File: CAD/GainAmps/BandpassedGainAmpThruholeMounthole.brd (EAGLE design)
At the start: 10.7 x 26.9 mm, 9 parts, among them U1 OPA202IDR

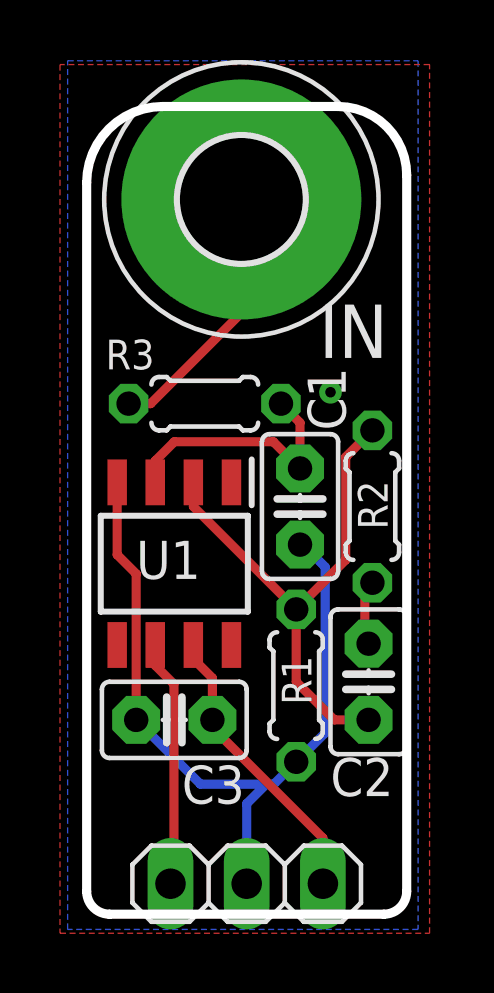
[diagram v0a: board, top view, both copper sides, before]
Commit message: fixes
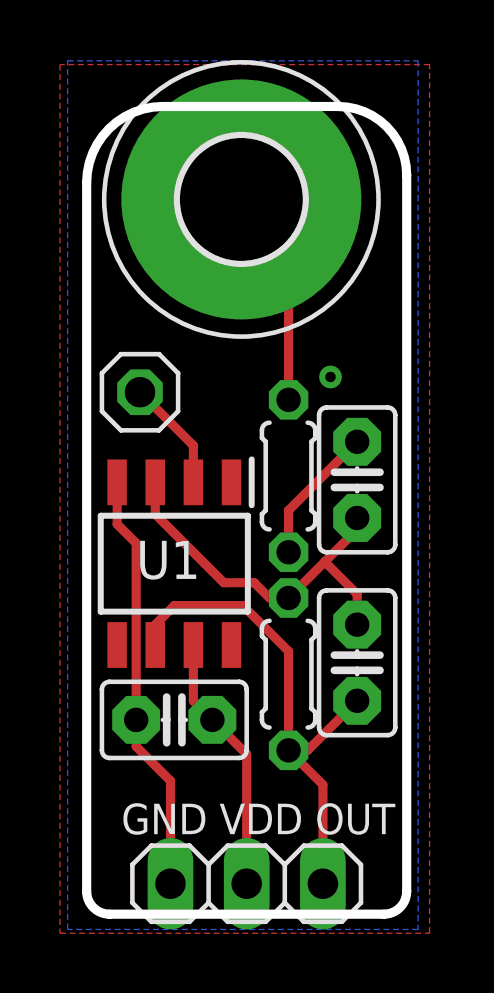
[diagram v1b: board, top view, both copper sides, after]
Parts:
- removed R3: 1K, rcl:0204/5
- added REF: (no value), pinhead:1X01
- moved R1 6.99 mm to (7.75, 17.7), turned to 270 degrees
- moved R2 6.25 mm to (7.75, 11.0)
- moved C1 2.10 mm to (10.0, 17.5), turned to 270 degrees
- moved C2 0.74 mm to (10.0, 11.4), turned to 270 degrees
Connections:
- removed net -IN: C2.1, R1.2, R2.1, U1.2
- removed net N$3: C2.2, R2.2
- new net +REF: REF.1, U1.2
- new net R1C1: C1.1, R1.2
- net +IN: now also C2.1, R2.1; no longer R3.2
- net GND: now also JP1.3; no longer C1.1, JP1.2, R1.1
- net IN: now also R1.1; no longer R3.1
- net OUT: now also C2.2, JP1.1, R2.2; no longer JP1.3
- net VDD: now also JP1.2; no longer JP1.1
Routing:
- net -IN: track 18.0 -> 0.00 mm
- net GND: track 26.3 -> 14.1 mm
- net OUT: track 8.29 -> 17.2 mm
- net R1C1: track 0.00 -> 4.63 mm
- net +IN: track 8.60 -> 12.8 mm
- net +REF: track 0.00 -> 3.74 mm
- net N$3: track 2.19 -> 0.00 mm
- net IN: track 8.80 -> 7.33 mm
- net VDD: track 9.75 -> 9.16 mm
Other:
- board text added: "GND VDD OUT"
- board text removed: "VDD GND OUT"
